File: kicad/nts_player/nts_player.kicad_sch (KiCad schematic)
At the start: 95 parts, among them J1 SJ1-3523N, J2 RCJ-2123, SW1 PEC11R-4120F-S0018, U1 ESP32-S3-DEV-KIT-N16R8, U2 LM66100DCKR, U3 TPS7A2033PDBVR, U4 TPS22918DBVR, U5 SN74AHCT1G125DBVR, U6 PCM5122PWR

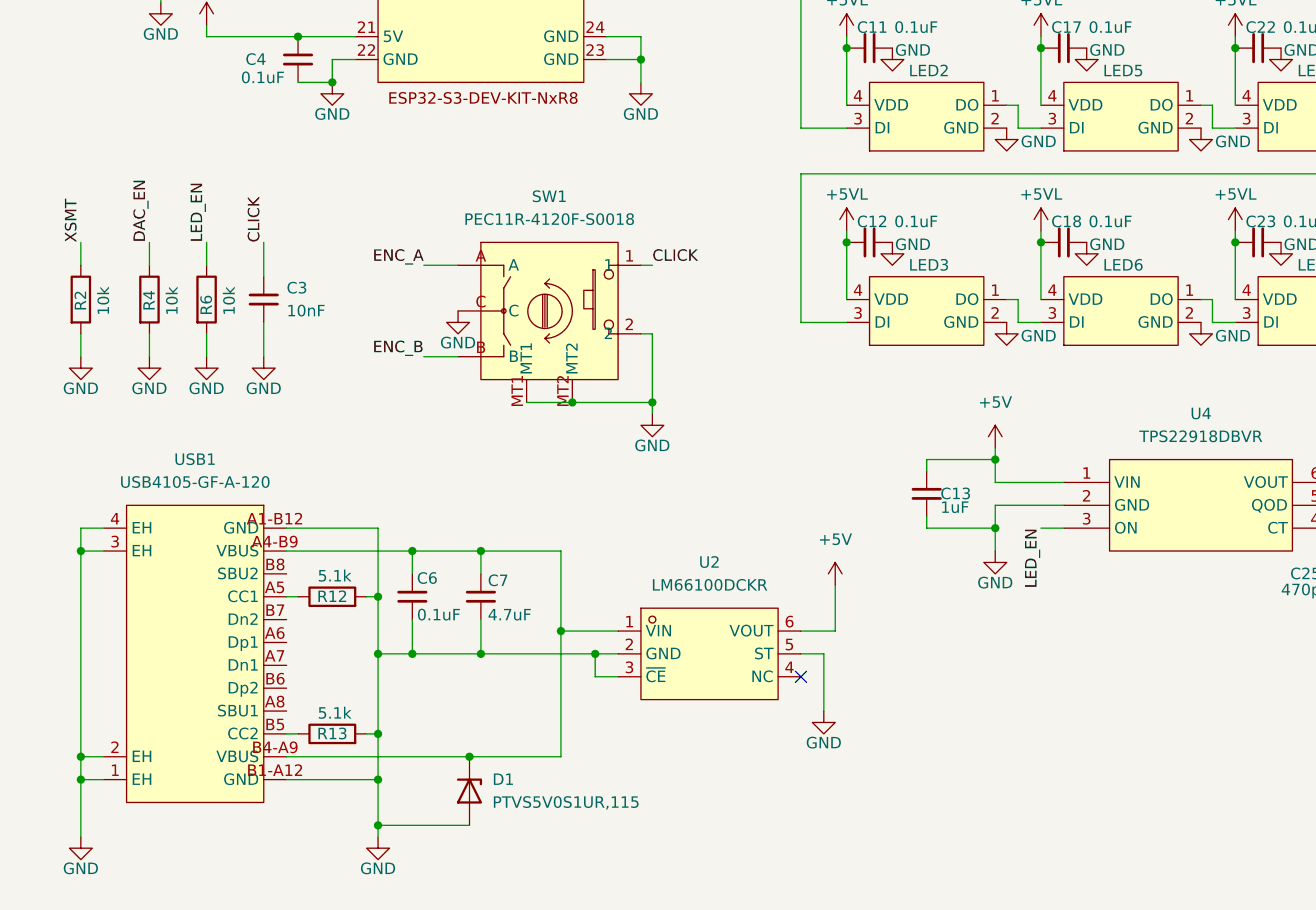
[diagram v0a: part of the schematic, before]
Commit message: feat: change usb
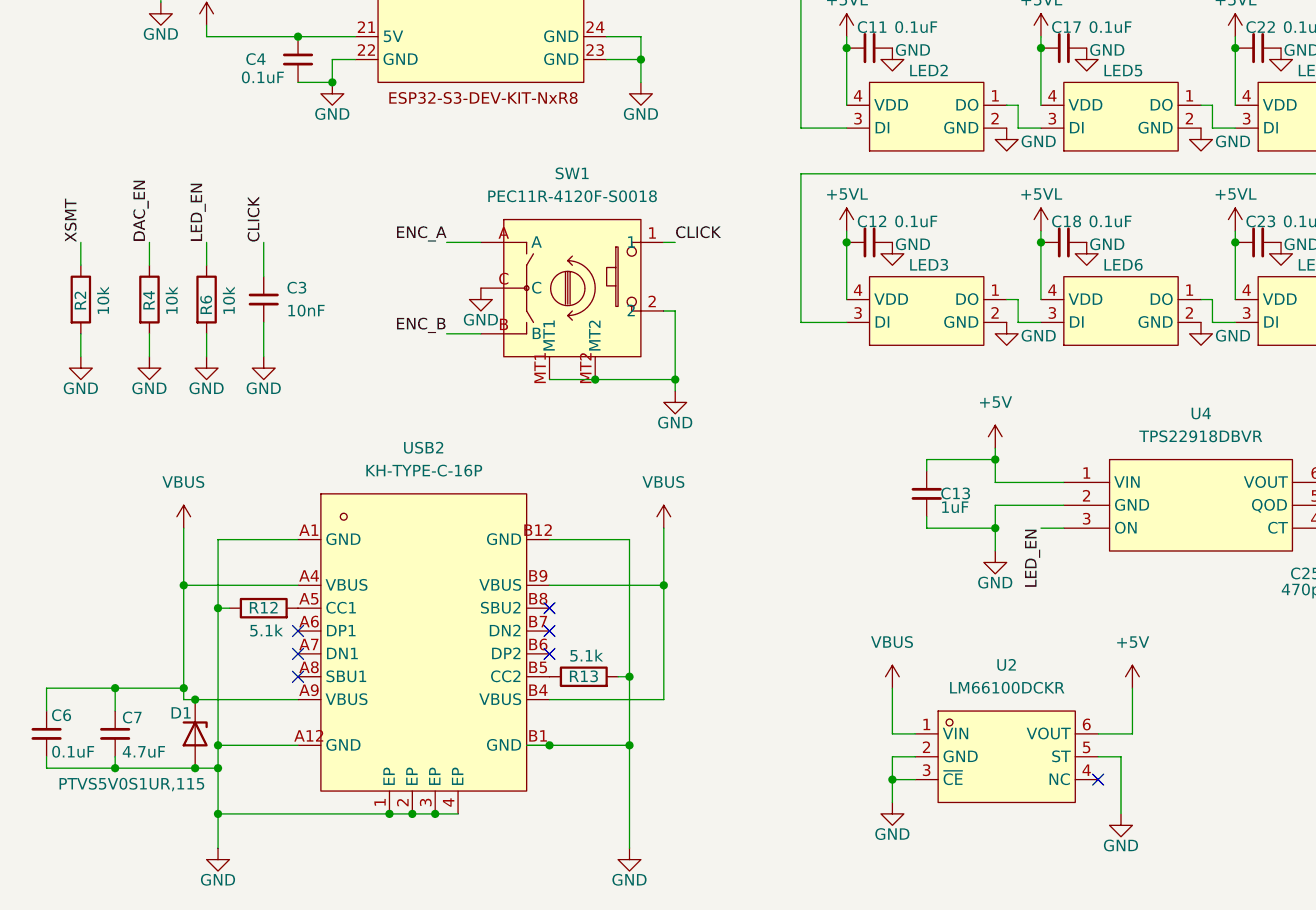
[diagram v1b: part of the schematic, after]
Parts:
- removed USB1: USB4105-GF-A-120, lcsc:USB-C-SMD_MC-311D, symbol lcsc:USB4105-GF-A-120
- added USB2: KH-TYPE-C-16P, lcsc:USB-C-SMD_KH-TYPE-C-16P, symbol lcsc:KH-TYPE-C-16P
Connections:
- net GND: now also R12.1, USB2.1 (EP), USB2.2 (EP), USB2.3 (EP), USB2.4 (EP), USB2.A1 (GND), USB2.A12 (GND), USB2.B1 (GND), USB2.B12 (GND); no longer R12.2
- net VBUS: now reaches C6.2, C7.1, D1.1 (K), U2.1 (VIN)
- net VBUS: now also USB2.A4 (VBUS), USB2.A9 (VBUS), USB2.B4 (VBUS), USB2.B9 (VBUS)
- net at R13.1: now also USB2.B5 (CC2)
- new net: R12.2, USB2.A5 (CC1)
- no-connect marks 29 -> 35
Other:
- moved on the sheet: SW1, U2
